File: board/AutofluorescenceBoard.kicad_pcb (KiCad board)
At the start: 2 copper layers, 40 parts, among them J1 2002411212, Q1 BSS138, U1 PAM2863ECR, U2 PAM2863ECR, U3 PAM2863ECR

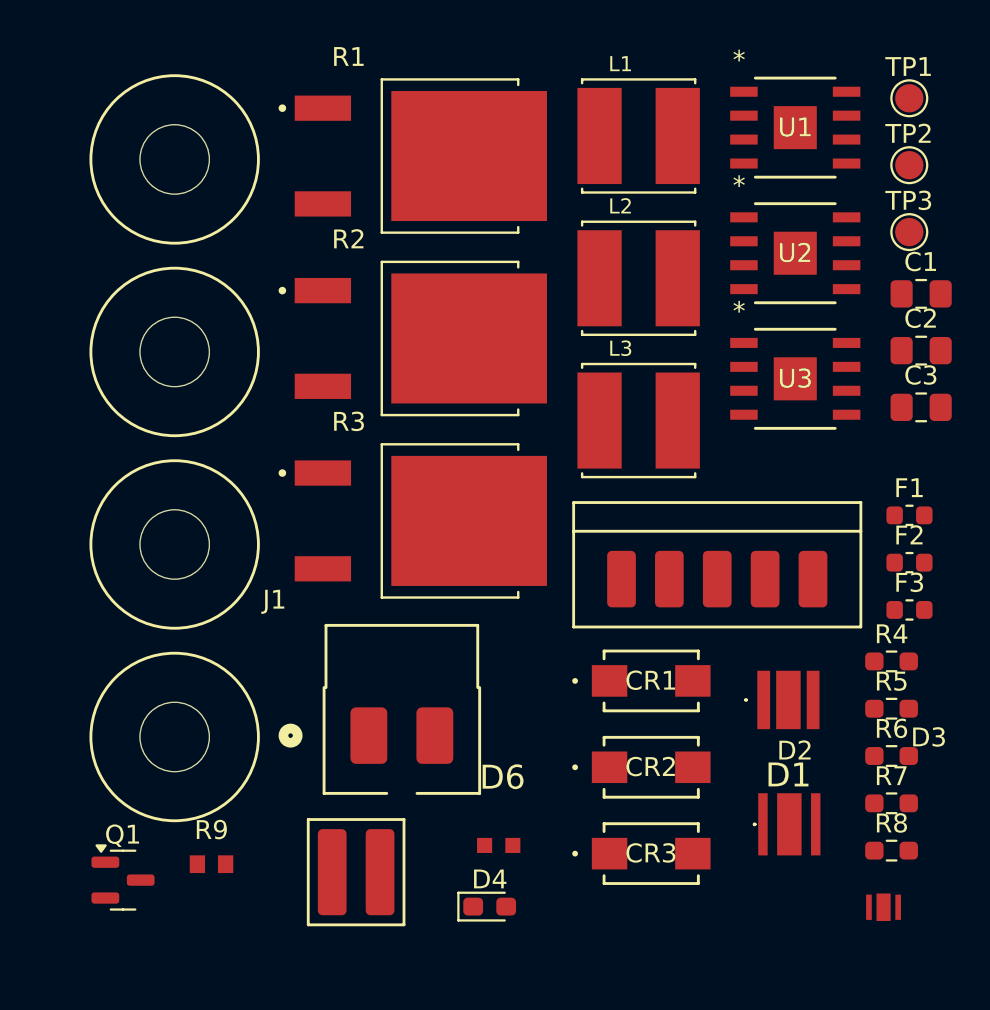
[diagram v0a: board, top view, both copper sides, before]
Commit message: Rev2 Initial Component Placement
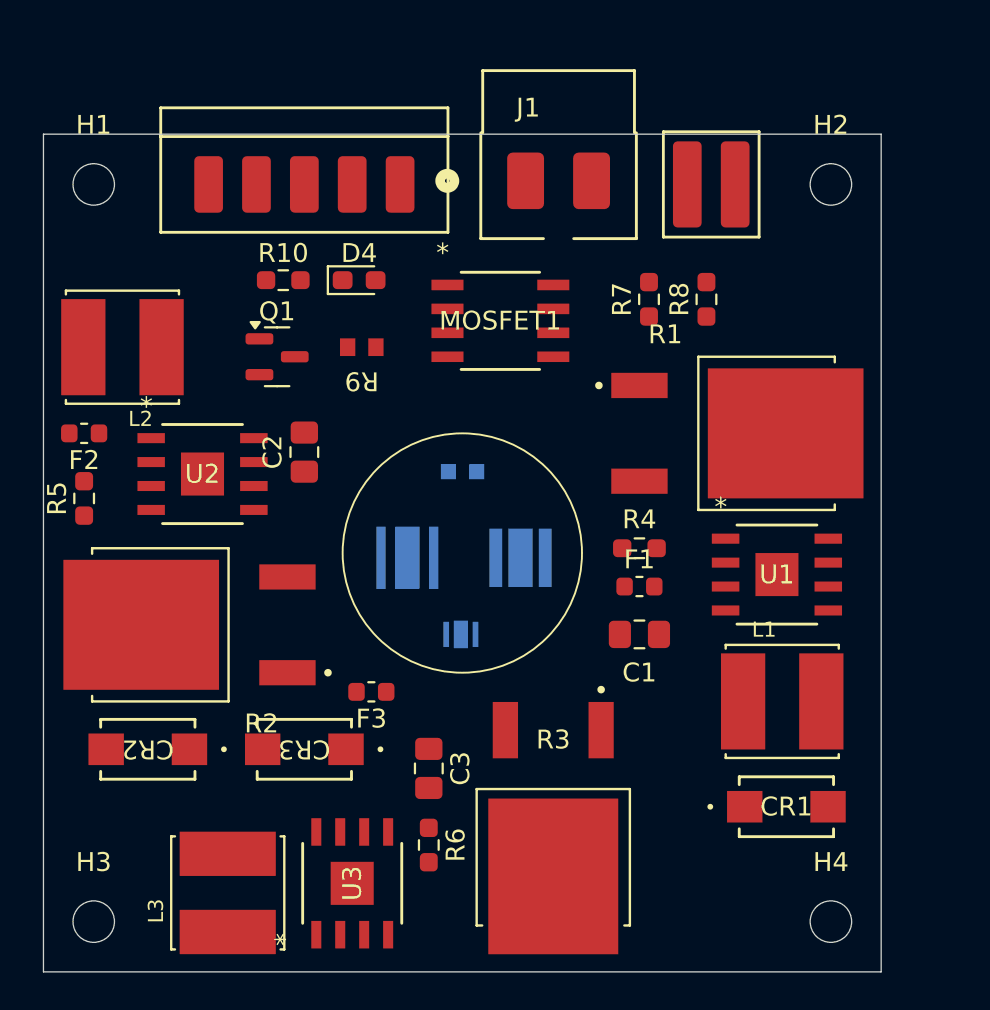
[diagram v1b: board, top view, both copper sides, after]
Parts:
- removed TP1, TP2, TP3: TestPoint, TestPoint:TestPoint_Pad_D1.5mm
- added MOSFET1: TPC8132_LQS, AutofluorescenceBoard:SOP-8_TOS-M, F.Cu at (146.5, 81.4)
- added R10: 10K, Resistor_SMD:R_0603_1608Metric_Pad0.98x0.95mm_HandSolder, F.Cu at (135.0, 79.2)
- D1, D2, D3, D6: moved to B.Cu
- H1, H2, H3, H4: footprint MRDT_Drill_Holes:6_32_Hole_Corner -> MountingHole:MountingHole_2.2mm_M2
- moved F2 44.3 mm to (124.5, 87.4), turned to 180 degrees
- moved R5 44.3 mm to (124.5, 90.8), turned to 90 degrees
- moved H2 41.5 mm to (164.1, 74.2)
- moved FanConn1 41.1 mm to (156.5, 72.6)
- moved H4 39.6 mm to (164.1, 113.3)
- moved U3 35.6 mm to (138.7, 111.3), turned to 90 degrees
- moved D4 34.0 mm to (139.1, 79.2)
- moved U2 33.6 mm to (130.7, 89.5)
- moved L3 33.2 mm to (132.1, 111.8), turned to 90 degrees
- moved C2 33.2 mm to (136.1, 88.4), turned to 90 degrees
- moved C3 32.4 mm to (142.7, 105.2), turned to -90 degrees
- moved L1 31.0 mm to (161.5, 101.6)
- moved R8 30.9 mm to (157.5, 80.3), turned to 90 degrees
- moved J1 30.6 mm to (147.9, 74.0)
- moved Conn1 30.3 mm to (131.1, 74.2)
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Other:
- board outline added: 44.5 x 44.4 mm
- copper layers 2 -> 4
